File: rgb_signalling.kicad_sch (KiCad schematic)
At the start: 7 parts, among them IC1 TXB0108PWR

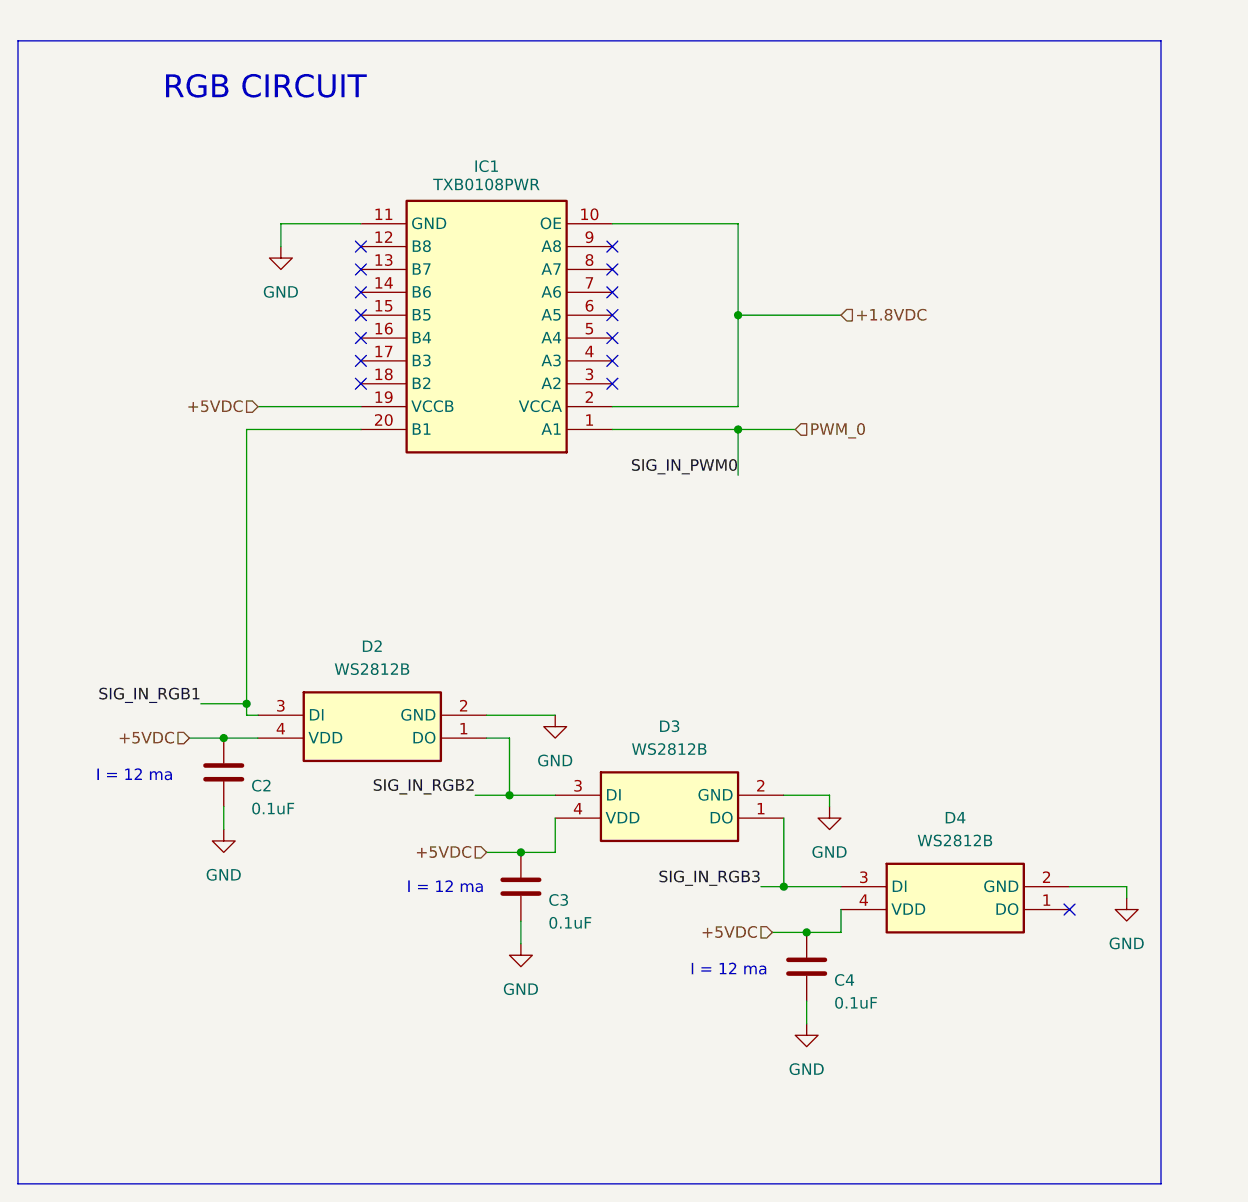
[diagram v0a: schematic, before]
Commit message: latest updates, up to v2
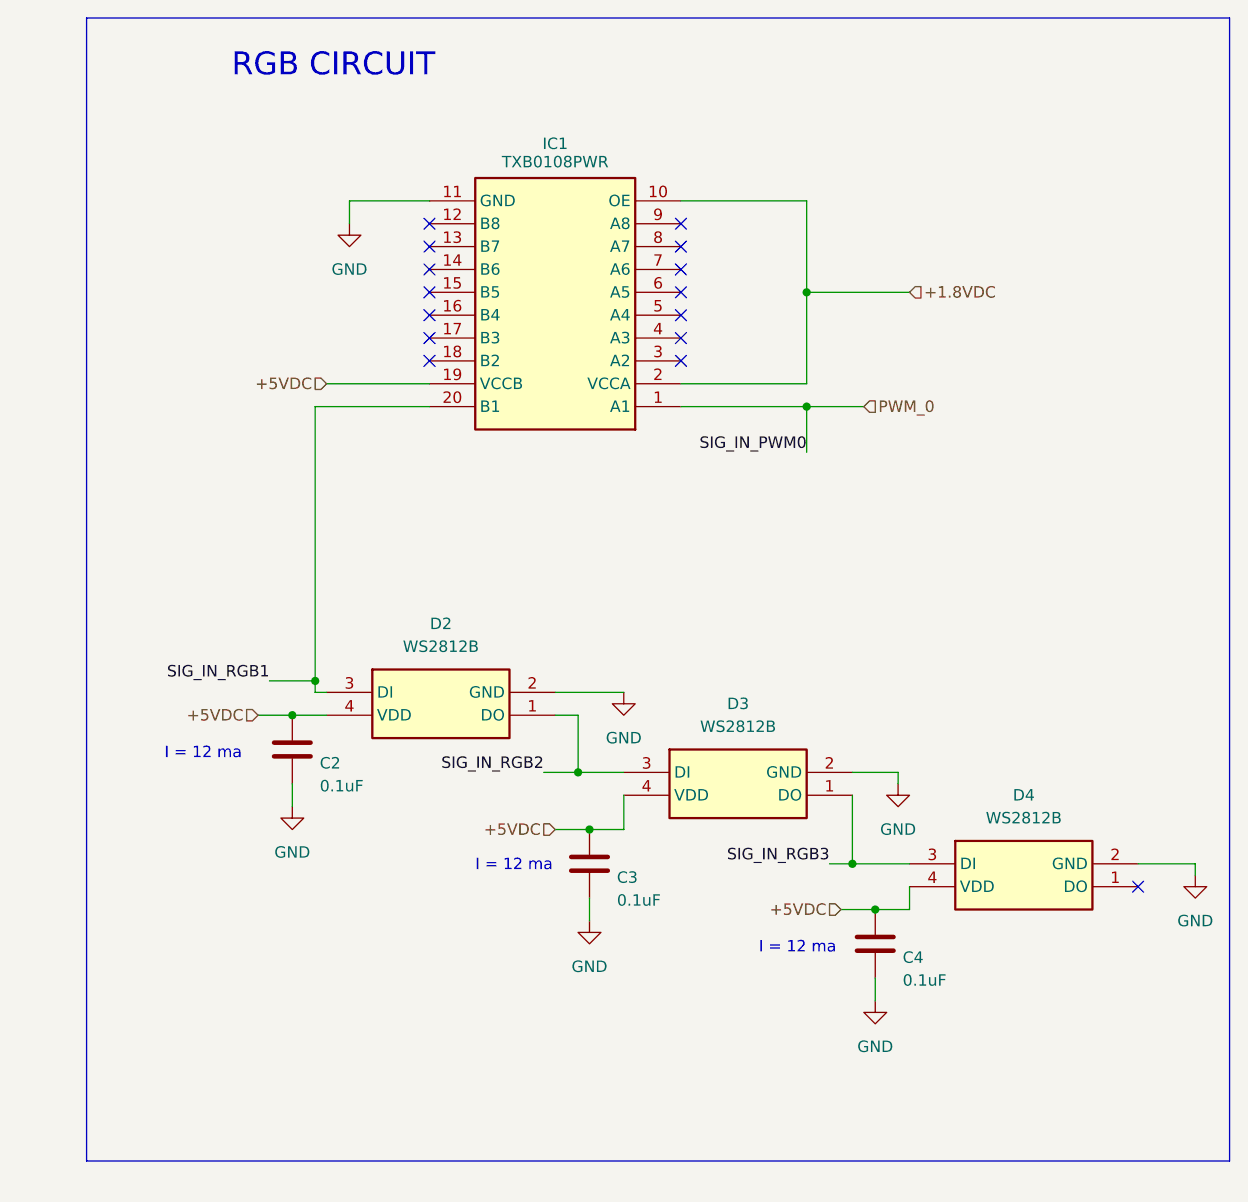
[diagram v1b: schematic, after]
